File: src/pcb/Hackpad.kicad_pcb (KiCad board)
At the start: 2 copper layers, 79 x 47.3 mm, 7 parts, among them SW1 SW_Push, SW2 SW_Push, SW3 SW_Push, SW4 SW_Push, U1 XIAO-RP2040-DIP

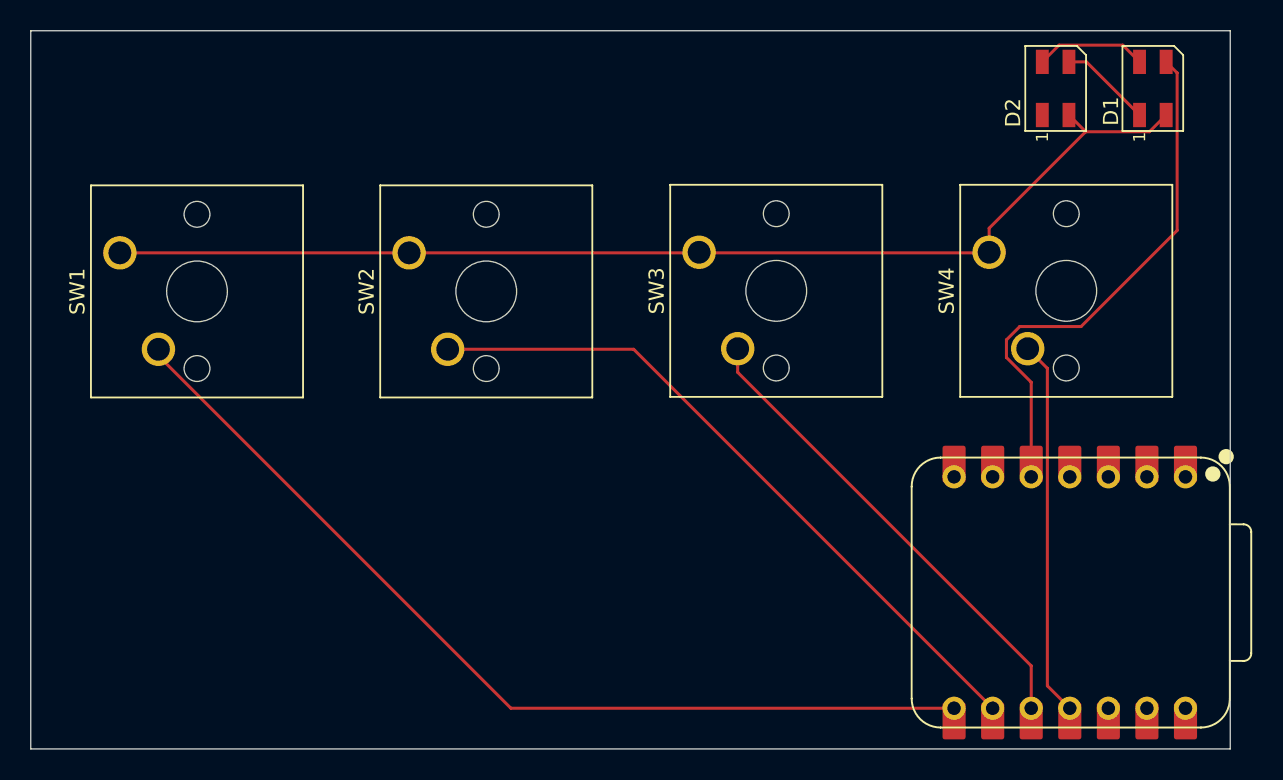
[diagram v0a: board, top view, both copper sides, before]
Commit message: gnd fill
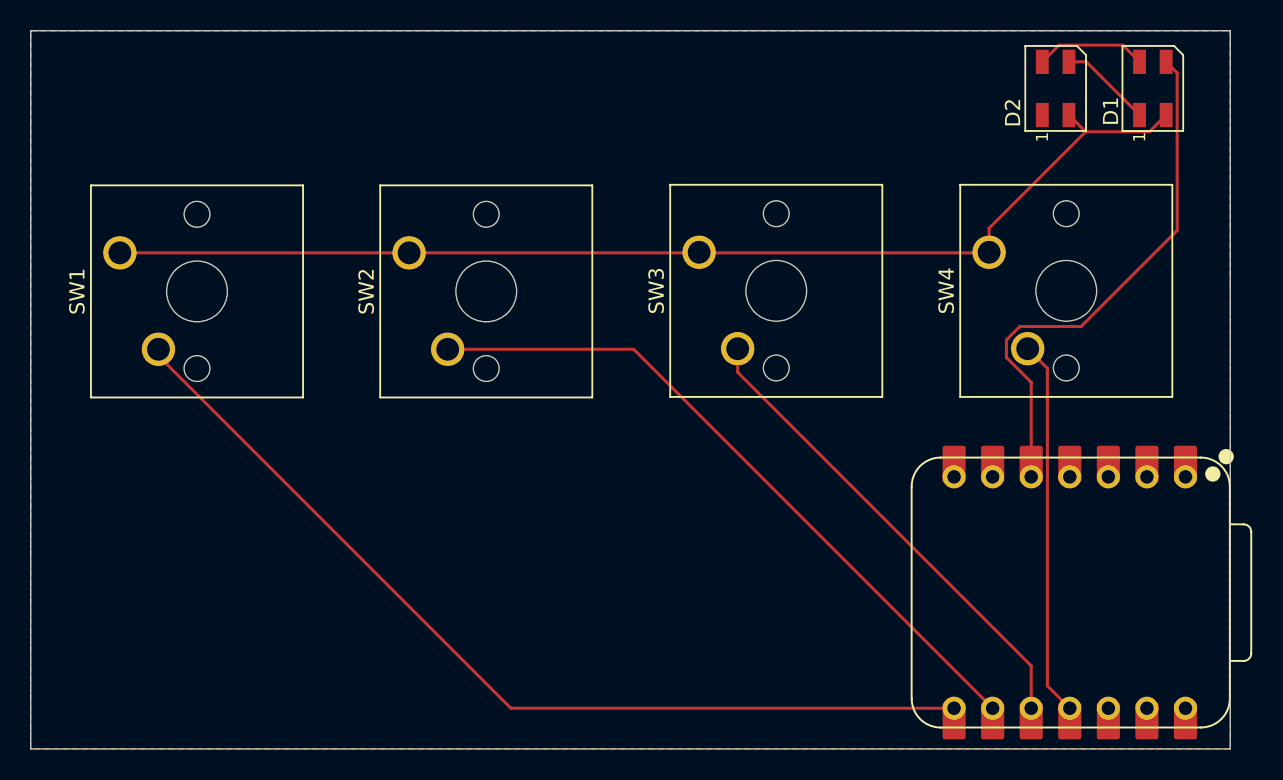
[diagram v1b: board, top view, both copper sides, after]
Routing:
- added copper zone on F.Cu, net GND
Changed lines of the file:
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@@
 		(net 8)
+	)
+	(zone
+		(net 4)
+		(net_name "GND")
+		(layer "F.Cu")
+		(hatch edge 0.5)
+		(connect_pads
+			(clearance 0.5)
+		)
+		(min_thickness 0.25)
+		(filled_areas_thickness no)
+		(fill
+			(thermal_gap 0.5)
+			(thermal_bridge_width 0.5)
+		)
+		(polygon
+			(pts
+				(xy 110.89 64.21) (xy 110.9 111.5) (xy 31.9 111.5) (xy 31.92 64.22)
+			)
+		)
 	)
 	(embedded_fonts no)
